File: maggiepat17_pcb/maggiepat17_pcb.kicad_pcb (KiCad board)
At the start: 2 copper layers, 110 x 38.3 mm, 55 parts, among them J1 USB_C_Receptacle, J2 AudioJack4, J3 Conn_01x03_Male, J4 Conn_01x03_Male, J5 TP1, J6 TP2, J7 TP3, SW1 SW_Push, SW10 RESET, SW2 SW_Push, SW3 SW_Push, SW4 SW_Push, SW5 SW_Push, SW6 SW_Push, SW7 SW_Push, SW8 SW_Push, SW9 BOOT, U1 NCP1117-3.3_SOT223, U2 RP2040, U3 W25Q128JVSIQ, Y1 12MHz

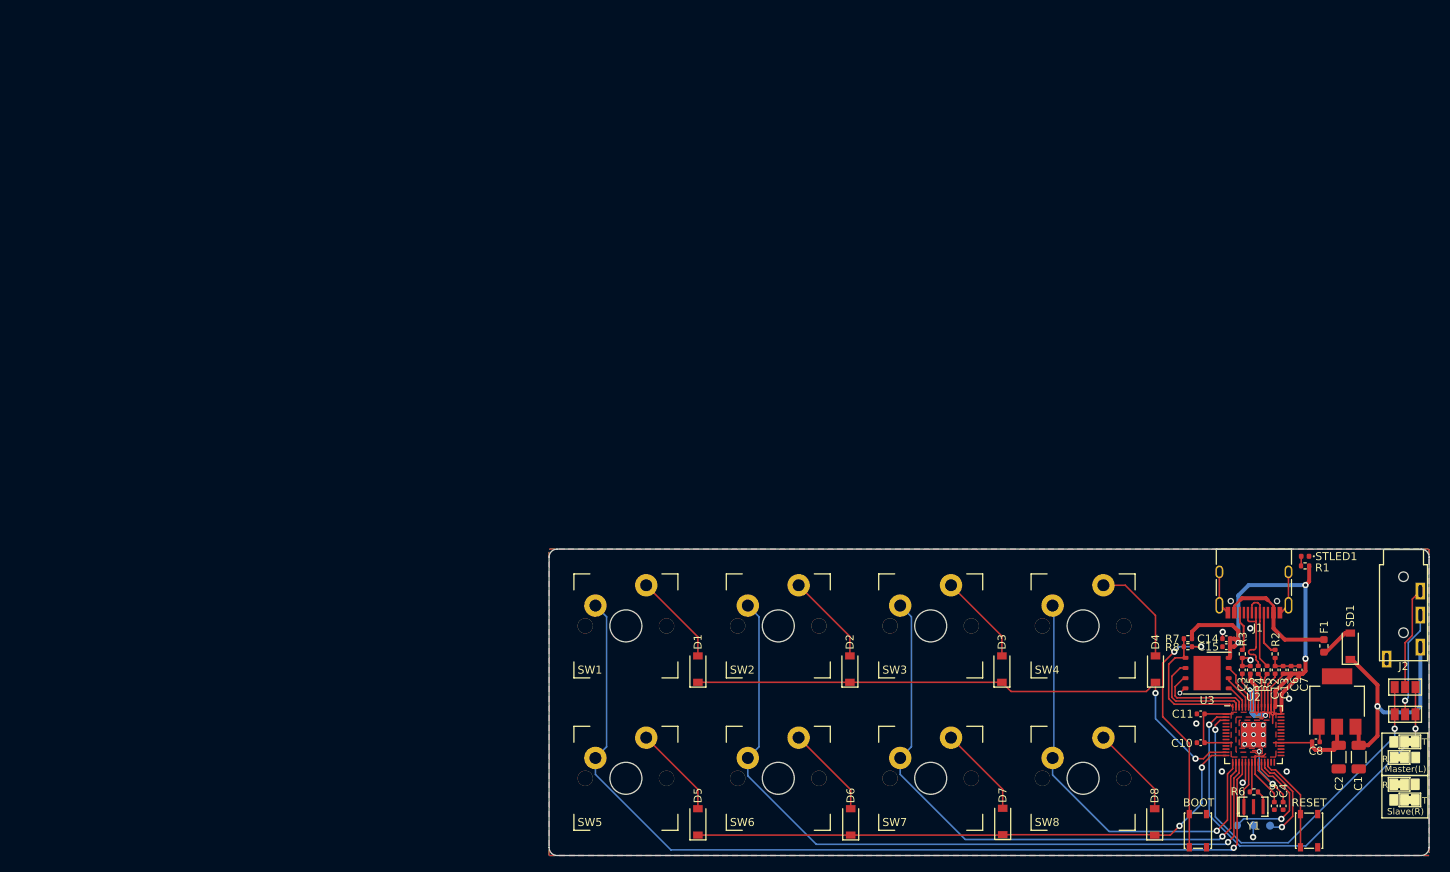
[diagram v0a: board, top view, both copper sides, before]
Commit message: created PCBA order files, need to replace
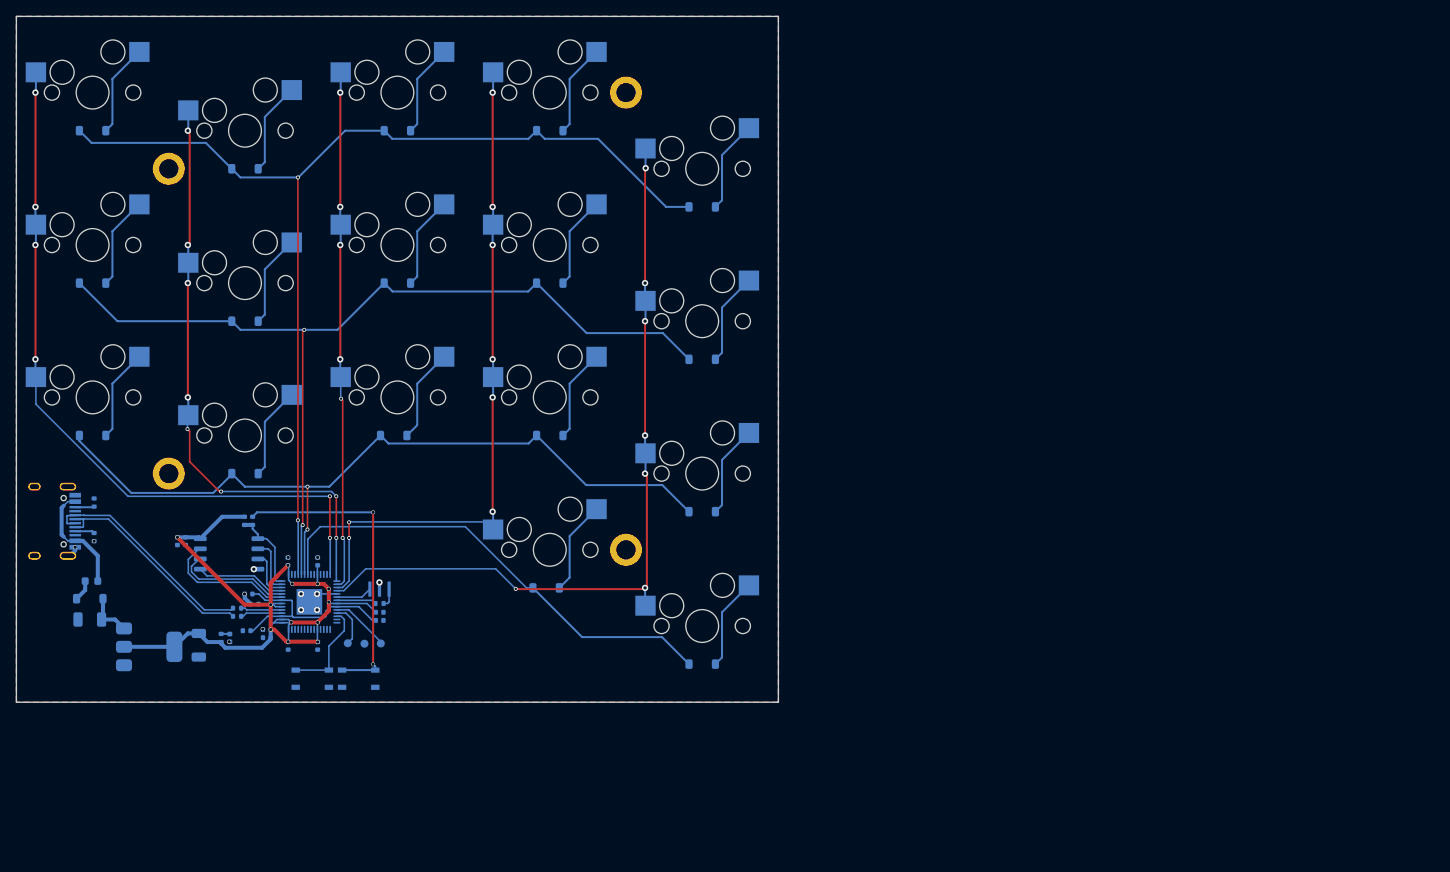
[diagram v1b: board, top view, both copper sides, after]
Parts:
- removed J2: AudioJack4, yuchi_kbd:PJ-320
- removed J3, J4: Conn_01x03_Male, Jumper:SolderJumper-3_P1.3mm_Open_Pad1.0x1.5mm_NumberLabels
- added D10: D_Small, Diode_SMD:D_SOD-123, B.Cu at (109.5, 66.7)
- added D11: D_Small, Diode_SMD:D_SOD-123, B.Cu at (33.3, 76.2)
- added D12: D_Small, Diode_SMD:D_SOD-123, B.Cu at (52.4, 81.0)
- added D13: D_Small, Diode_SMD:D_SOD-123, B.Cu at (71.0, 76.2)
- added D14: D_Small, Diode_SMD:D_SOD-123, B.Cu at (90.5, 76.2)
- added D15: D_Small, Diode_SMD:D_SOD-123, B.Cu at (109.5, 85.7)
- added D16: D_Small, Diode_SMD:D_SOD-123, B.Cu at (90.0, 95.2)
- added D17: D_Small, Diode_SMD:D_SOD-123, B.Cu at (109.5, 104.8)
- added D9: D_Small, Diode_SMD:D_SOD-123, B.Cu at (90.5, 57.1)
- added REF**: HOLE_M2_PCB, yuchi_kbd_lib:HOLE_M2_CASEPCB, F.Cu at (42.9, 81.0)
- added REF**: HOLE_M2_PCB, yuchi_kbd_lib:HOLE_M2_CASEPCB, F.Cu at (100.0, 90.5)
- added REF**: HOLE_M2_PCB, yuchi_kbd_lib:HOLE_M2_CASEPCB, F.Cu at (42.9, 42.9)
- added REF**: HOLE_M2_PCB, yuchi_kbd_lib:HOLE_M2_CASEPCB, F.Cu at (100.0, 33.3)
- added SW11: SW_Push, kbd:keyswitch_cherrymx_hotswap_1u, B.Cu at (33.3, 71.4)
- added SW12: SW_Push, kbd:keyswitch_cherrymx_hotswap_1u, B.Cu at (52.4, 76.2)
- added SW13: SW_Push, kbd:keyswitch_cherrymx_hotswap_1u, B.Cu at (71.4, 71.4)
- added SW14: SW_Push, kbd:keyswitch_cherrymx_hotswap_1u, B.Cu at (90.5, 71.4)
- added SW15: SW_Push, kbd:keyswitch_cherrymx_hotswap_1u, B.Cu at (109.5, 81.0)
- added SW16: SW_Push, kbd:keyswitch_cherrymx_hotswap_1u, B.Cu at (90.5, 90.5)
- added SW17: SW_Push, kbd:keyswitch_cherrymx_hotswap_1u, B.Cu at (109.5, 100.0)
- added SW_BOOT1: BOOT, Button_Switch_SMD:SW_SPST_PTS810, B.Cu at (66.6, 106.6)
- added SW_RESET1: RESET, Button_Switch_SMD:SW_SPST_PTS810, B.Cu at (60.8, 106.6)
- C1, C10, C11, C12, C13, C14, C15, C2, C3, C4, C5, C6, C7, C8, C9, D1, D2, D3, D4, D5, D6, D7, D8, F1, J1, R1, R2, R3, R4, R5, R6, R7, R8, SD1, STLED1, U2, Y1: moved to B.Cu
- SW1, SW2, SW3, SW4, SW5, SW6, SW7, SW8: footprint yuchi:MX_HOLE -> kbd:keyswitch_cherrymx_hotswap_1u; moved to B.Cu
- SW10: value RESET -> SW_Push; footprint Button_Switch_SMD:SW_SPST_PTS810 -> kbd:keyswitch_cherrymx_hotswap_1u; moved to B.Cu
- SW9: value BOOT -> SW_Push; footprint Button_Switch_SMD:SW_SPST_PTS810 -> kbd:keyswitch_cherrymx_hotswap_1u; moved to B.Cu
- U1: footprint Package_TO_SOT_SMD:SOT-223 -> Package_TO_SOT_SMD:SOT-223-3_TabPin2; moved to B.Cu
- U3: footprint Package_SON:WSON-8-1EP_6x5mm_P1.27mm_EP3.4x4.3mm -> Package_SO:SOIC-8_5.23x5.23mm_P1.27mm; moved to B.Cu
- moved C1 159.5 mm to (33.0, 99.2), turned to 180 degrees
- moved SD1 157.7 mm to (33.0, 96.6), turned to 180 degrees
- moved F1 154.3 mm to (33.2, 94.4), turned to 180 degrees
- moved J1 151.6 mm to (27.1, 86.9), turned to 90 degrees
- moved R2 148.8 mm to (33.5, 84.6), turned to 90 degrees
- moved U1 148.6 mm to (40.4, 102.6), turned to 0 degrees
- moved R3 144.3 mm to (33.5, 88.9)
- moved C2 143.2 mm to (46.6, 102.4)
- moved R1 135.8 mm to (49.4, 101.5), turned to -90 degrees
- moved STLED1 134.8 mm to (50.5, 101.5), turned to 90 degrees
- moved C4 132.0 mm to (52.8, 96.0), turned to 180 degrees
- moved C14 131.7 mm to (43.9, 89.4), turned to -90 degrees
- moved C15 130.8 mm to (45.0, 89.4), turned to -90 degrees
- moved C9 129.9 mm to (53.6, 97.3), turned to 180 degrees
- moved C7 129.1 mm to (55.1, 101.5), turned to 180 degrees
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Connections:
- net rotary renamed Net-(D4-A)
- D5 pad 1: row1 -> row0
- R2 pad 1: Net-(J1-CC1) -> Net-(J1-CC2)
- R3 pad 1: Net-(J1-CC2) -> Net-(J1-CC1)
- SW10 pad 1: RESET -> col4
- SW10 pad 2: GND -> Net-(D10-A)
- SW5 pad 1: col0 -> col4
- SW6 pad 1: col1 -> col0
- SW7 pad 1: col2 -> col1
- SW8 pad 1: col3 -> col2
- SW9 pad 1: USB_BOOT -> col3
- SW9 pad 2: GND -> Net-(D9-A)
- U2 pad 13: row0 -> unconnected-(U2-GPIO10-Pad13)
- U2 pad 14: row1 -> col0
- U2 pad 15: col3 -> col1
- U2 pad 17: col1 -> col3
- U2 pad 18: col0 -> col4
- U2 pad 2: TX -> unconnected-(U2-GPIO0-Pad2)
- U2 pad 3: RX -> unconnected-(U2-GPIO1-Pad3)
- U2 pad 4: unconnected-(U2-GPIO2-Pad4) -> row0
- U2 pad 5: unconnected-(U2-GPIO3-Pad5) -> row1
- U2 pad 6: unconnected-(U2-GPIO4-Pad6) -> row2
- U2 pad 7: unconnected-(U2-GPIO5-Pad7) -> row3
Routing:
- net row2: track 0.00 -> 99.9 mm, vias 0 -> 2
- net col4: track 0.00 -> 98.0 mm, vias 0 -> 7
- net row0: track 73.9 -> 135.5 mm
- net row3: track 0.00 -> 59.8 mm
- net TX: track 53.0 -> 0.00 mm, vias 2 -> 0
- net RX: track 48.5 -> 0.00 mm, vias 2 -> 0
- net row1: track 73.0 -> 116.6 mm
- net col3: track 54.2 -> 84.8 mm, vias 1 -> 8
- net col0: track 117.2 -> 92.7 mm, vias 1 -> 6
- net +5V: track 29.8 -> 5.93 mm, vias 1 -> 0
- net col1: track 96.7 -> 75.1 mm, vias 1 -> 8
- net GND: track 27.5 -> 7.40 mm, vias 19 -> 13
- net D-: track 10.2 -> 27.9 mm
- net D+: track 10.1 -> 27.7 mm
- net R1: track 13.2 -> 0.00 mm, vias 1 -> 0
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- removed copper zone on F.Cu, net +1V1
- removed copper zone on F.Cu, net +3V3
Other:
- board size 110 x 38.3 mm -> 95.2 x 85.7 mm
- board text removed: "IO28 IO27"
- board text removed: "Master(L)"
- board text removed: "R"
- board text removed: "Slave(R)"
- board text removed: "T"
